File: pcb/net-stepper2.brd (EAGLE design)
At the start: 41.9 x 90.2 mm, 42 parts, among them J1 MICRO-USB, J2 POWER_JACKPTH_LOCK, J3 ENCODER, J4 ENDSTOP2, J5 ENDSTOP1, J6 STEPER, Q1 600mA/40V, Q2 600mA/40V, U1 L6470, U2 CP2104, U3 RGB-LED, U4 TRACO12433, U5 ESP-WROOM-32

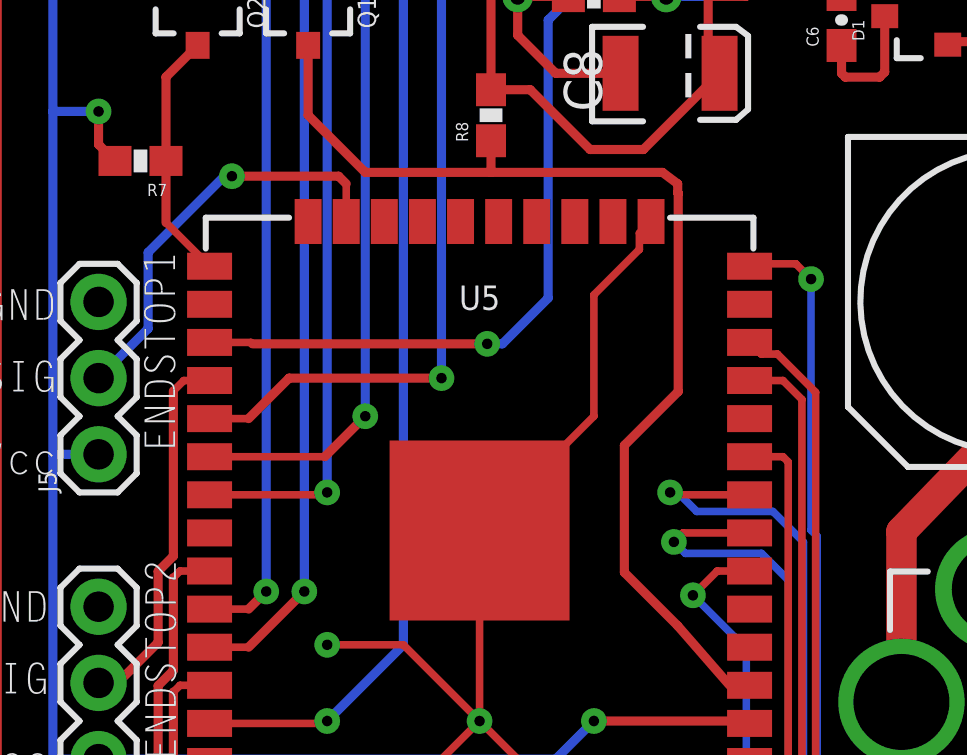
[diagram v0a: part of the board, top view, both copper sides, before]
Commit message: remapped pins
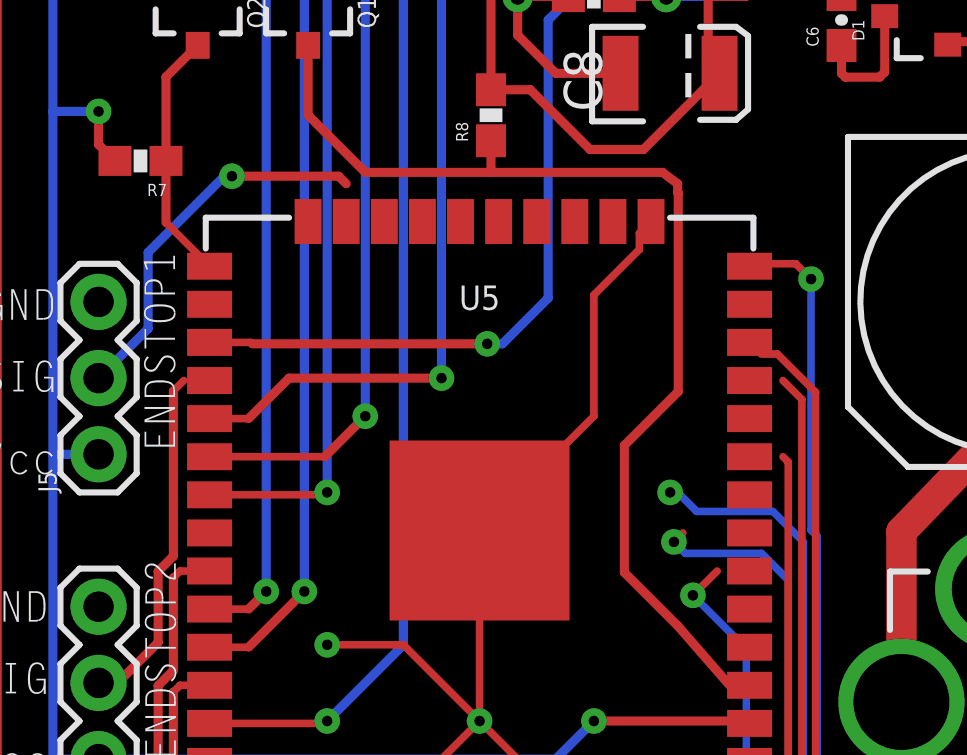
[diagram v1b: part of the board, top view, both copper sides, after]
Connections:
- net ADC renamed SC_ADC
- net CSN renamed SC_CSN
- net DTR renamed ESP_DTR
- net OUT1A renamed SC_OUT1A
- net OUT1B renamed SC_OUT1B
- net OUT2A renamed SC_OUT2A
- net OUT2B renamed SC_OUT2B
- net PGRM renamed ESP_PGRM
- net RESET renamed ESP_RESET
- net RESETN renamed SC_RESETN
- net RTS renamed ESP_RTS
- net RX renamed ESP_RX
- net SCK renamed SC_SCK
- net SDI renamed SC_SDI
- net SDO renamed SC_SDO
- net TX renamed ESP_TX
- removed net BLUE: R12.2, U2.13, U5.7
- removed net DOWN: S1.P$1, U5.11
- removed net END_STOP_1: J5.2, U5.23
- removed net END_STOP_2: J4.2, U5.28
- removed net GREEN: R11.2, U2.14, U5.6
- removed net HOME: S4.P$1, U5.12
- removed net RED: R6.2, U5.8
- removed net STOP: S3.P$1, U5.14
- removed net UP: S2.P$1, U5.9
- new net BTN_DOWN: S1.P$1, U5.26
- new net BTN_HOME: S4.P$1, U5.16
- new net BTN_STOP: S3.P$1, U5.23
- new net BTN_UP: S2.P$1, U5.10, U5.28
- new net ENDS_1: J5.2, U5.8
- new net ENDS_2: J4.2, U5.9
- new net LED_BLUE: R12.2, U2.13, U5.13
- new net LED_GREEN: R11.2, U2.14, U5.12
- new net LED_RED: R6.2, U5.11
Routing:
- net BLUE: track 110.9 -> 0.00 mm, vias 2 -> 0
- net LED_BLUE: track 0.00 -> 108.7 mm, vias 0 -> 2
- net GREEN: track 105.0 -> 0.00 mm, vias 2 -> 0
- net LED_GREEN: track 0.00 -> 103.9 mm, vias 0 -> 2
- net DOWN: track 48.7 -> 0.00 mm
- net BTN_DOWN: track 0.00 -> 47.6 mm
- net STOP: track 44.6 -> 0.00 mm, vias 2 -> 0
- net BTN_STOP: track 0.00 -> 44.5 mm, vias 0 -> 2
- net HOME: track 41.3 -> 0.00 mm
- net BTN_HOME: track 0.00 -> 40.8 mm
- net UP: track 37.8 -> 0.00 mm
- net BTN_UP: track 0.00 -> 36.7 mm
- net RED: track 32.6 -> 0.00 mm, vias 2 -> 0
- net LED_RED: track 0.00 -> 30.1 mm, vias 0 -> 2
- net END_STOP_1: track 13.9 -> 0.00 mm, vias 1 -> 0
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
